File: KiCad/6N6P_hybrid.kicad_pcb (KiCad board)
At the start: 2 copper layers, 165.1 x 144.1 mm, 71 parts, among them J1 MID Select, J10 Screw_Terminal_01x03, J11 Screw_Terminal_01x01, J12 Screw_Terminal_01x01, J13 Screw_Terminal_01x01, J14 Screw_Terminal_01x01, J15 PSU ground, J16 Screw_Terminal_01x01, J17 center tap, J18 chassis, J2 Input, J3 MID Bypass, J4 Low boost, J5 PrePower, J6 Volume, J7 Hi Cut, J8 6N6P, J9 OT feedback, Q1 BC107, U1 LTC1151CN8, U2 LTC1151CN8

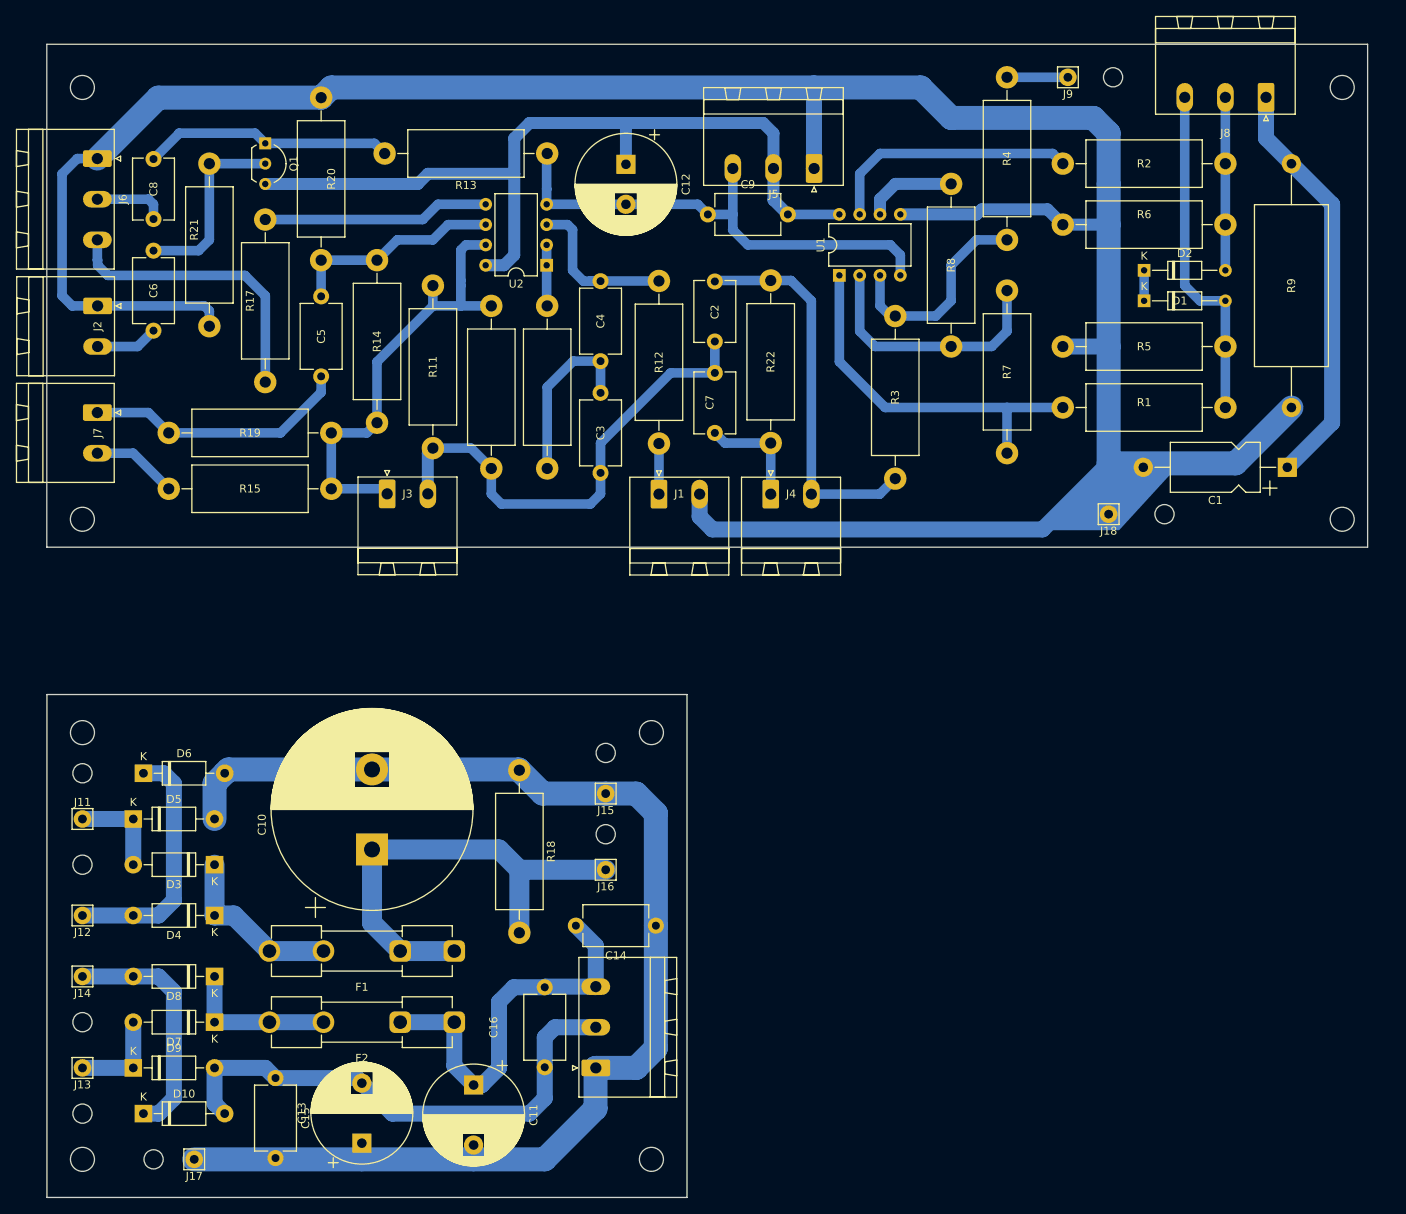
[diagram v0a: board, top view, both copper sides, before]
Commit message: Add files via upload
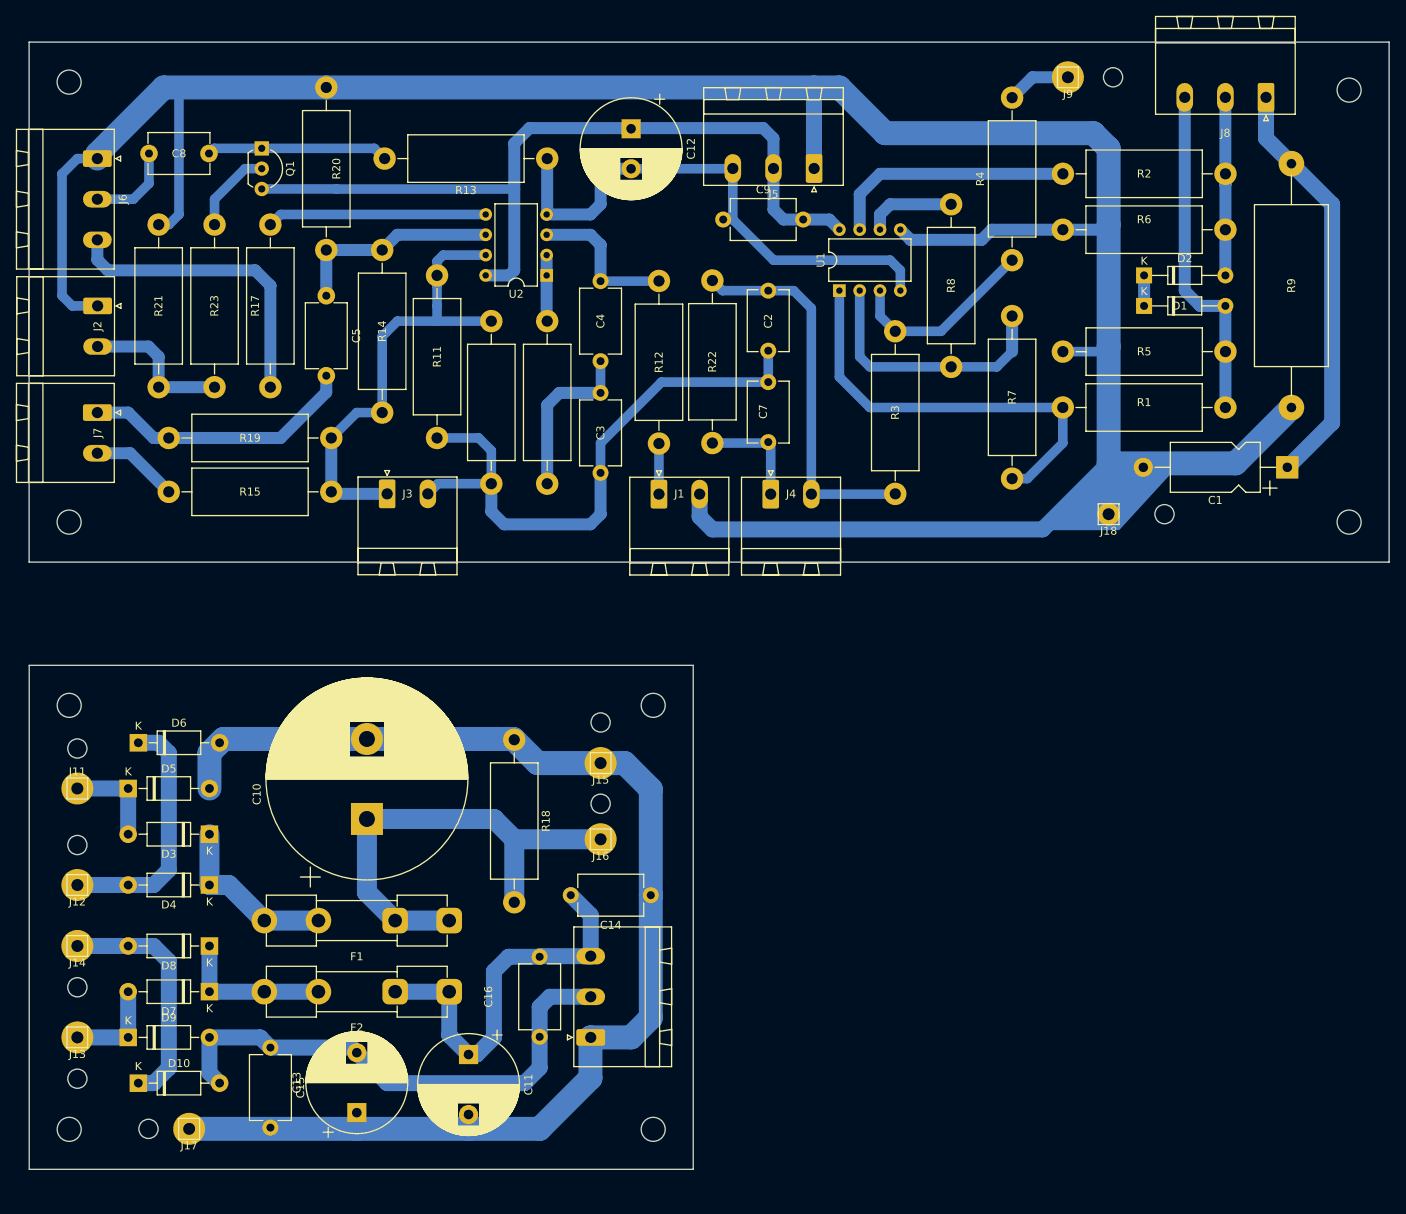
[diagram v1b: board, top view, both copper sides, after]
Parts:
- removed C6: 100n, Capacitor_THT:C_Disc_D8.0mm_W5.0mm_P10.00mm
- added R23: 10k, Resistor_THT:R_Axial_DIN0614_L14.3mm_D5.7mm_P20.32mm_Horizontal, F.Cu at (43.2, 43.8)
- moved R21 14.2 mm to (36.2, 43.8), turned to -90 degrees
- moved R22 7.29 mm to (105.4, 71.1)
- moved C8 6.97 mm to (42.5, 34.9), turned to 180 degrees
- moved C2 6.78 mm to (112.4, 59.6)
- moved C7 6.78 mm to (112.4, 63.5)
- moved C12 4.49 mm to (95.2, 31.8)
- moved D4 3.86 mm to (42.5, 126.4)
- moved J12 3.86 mm to (26.0, 126.4)
- moved C10 3.86 mm to (62.2, 118.1)
- moved C16 3.86 mm to (83.8, 145.3)
- moved D5 3.86 mm to (32.4, 114.3)
- moved D9 3.86 mm to (32.4, 145.4)
- moved F1 3.86 mm to (72.5, 130.8)
- moved F2 3.86 mm to (72.5, 139.7)
- moved J10 3.86 mm to (90.2, 145.4)
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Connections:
- R21 pad 2: Net-(Q1-B) -> Net-(J2-Pin_2)
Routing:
- net Net-(J3-Pin_2): track 61.2 -> 75.3 mm
- net Net-(Q1-B): track 24.1 -> 10.7 mm
- net Net-(J2-Pin_2): track 7.81 -> 19.0 mm
- net Net-(Q1-E): track 31.3 -> 22.8 mm
- net Net-(R1-Pad1): track 46.8 -> 53.6 mm
- net V--: track 62.7 -> 68.3 mm
- net V++: track 106.6 -> 103.2 mm
- net Net-(U1A-+): track 26.8 -> 24.2 mm
- net Net-(U2A-+): track 21.2 -> 19.1 mm
- net Net-(D2-A): track 21.6 -> 23.5 mm
- net Net-(J6-Pin_2): track 9.13 -> 11.0 mm
- net Net-(J6-Pin_3): track 36.5 -> 38.2 mm
- net GND: track 348.4 -> 349.7 mm
- net Net-(D1-A): track 41.5 -> 42.7 mm
- net Net-(J3-Pin_1): track 58.2 -> 59.3 mm
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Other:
- board size 165.1 x 144.1 mm -> 170 x 140.9 mm
